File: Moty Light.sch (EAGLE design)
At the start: 14 parts, among them T1 BTA16

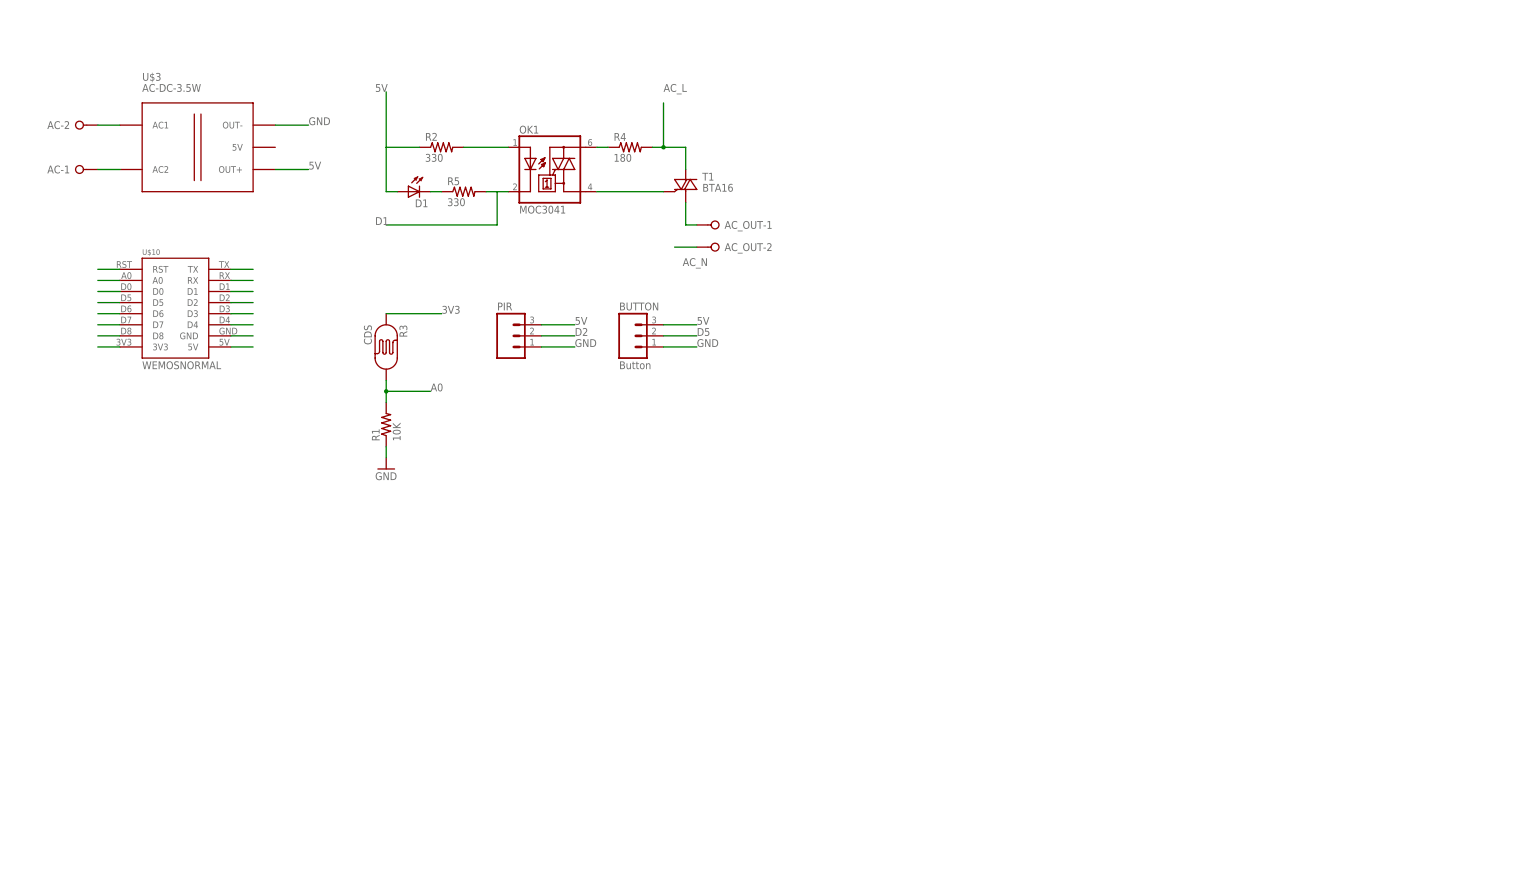
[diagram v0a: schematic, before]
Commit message: Update to version 0.2
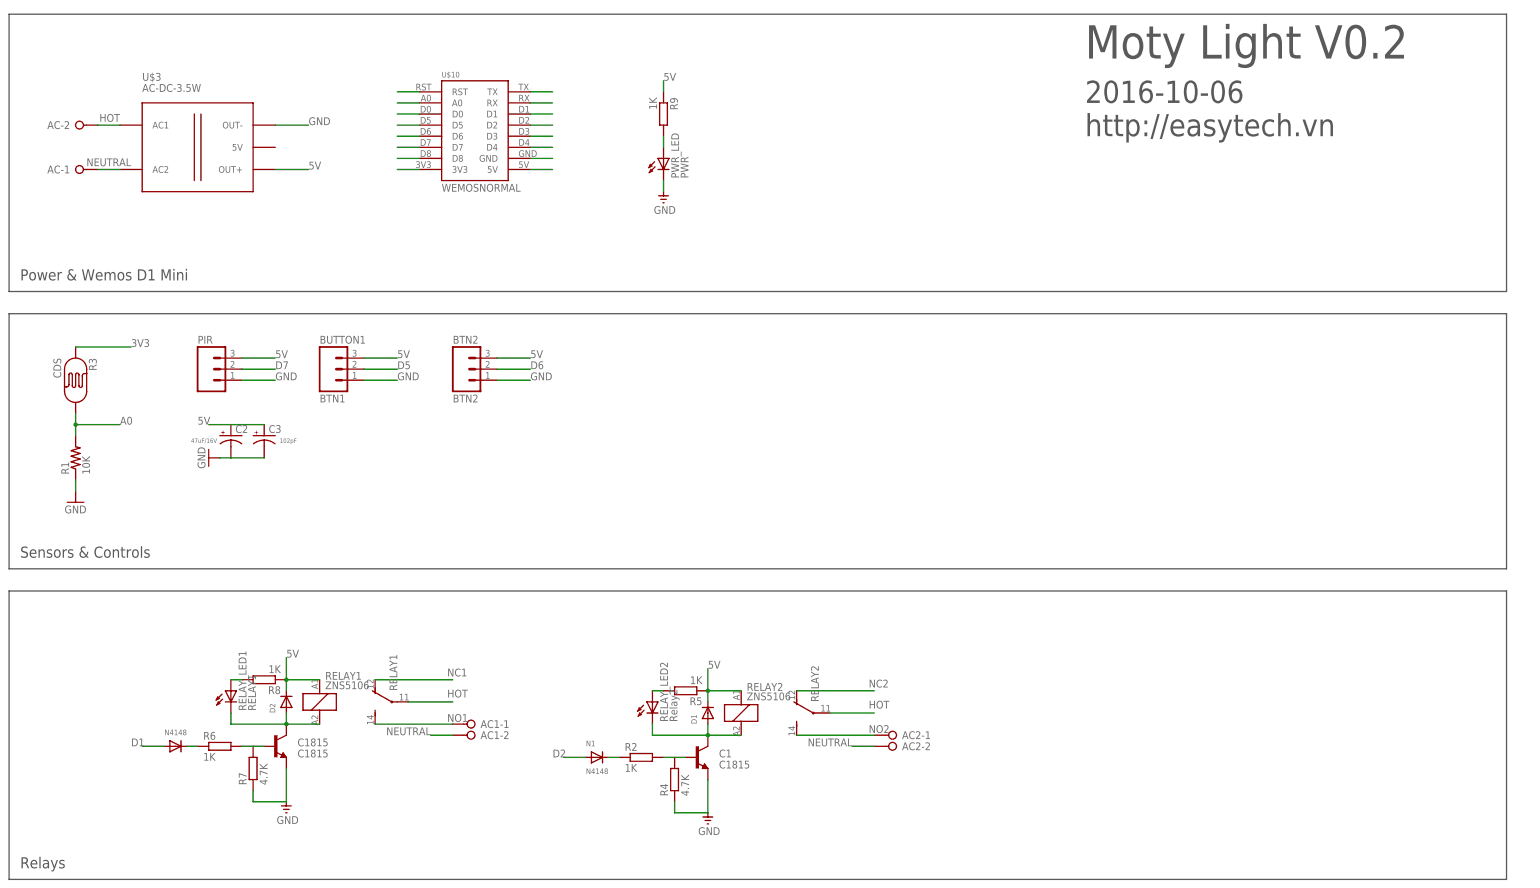
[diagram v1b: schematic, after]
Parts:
- removed AC_OUT: (no value), con-wago-508:W237-02P
- removed BUTTON: Button, SparkFun-Connectors:M03PTH
- removed OK1: MOC3041, optocoupler:MOC3032T
- removed T1: BTA16, triac:BT138-V
- added AC1, AC2: (no value), con-wago-508:W237-02P
- added BTN2: BTN2, SparkFun-Connectors:M03PTH
- added BUTTON1: BTN1, SparkFun-Connectors:M03PTH
- added C1, C1815: C1815, SparkFun-DiscreteSemi:TRANSISTOR_NPNSOT23-3
- added C2: 47uF/16V, SparkFun-Capacitors:CAP_POLPTH2
- added C3: 102pF, SparkFun-Capacitors:CAP_POLPTH2
- added D2: (no value), adafruit:DIODESMA
- added N1: N4148, adafruit:DIODESOD-123
- added N4148: (no value), adafruit:DIODESOD-123
- added PWR_LED: PWR, adafruit:LED3MM
- added R6, R8, R9: 1K, rcl:R-EU_R0805
- added R7: 4.7K, rcl:R-EU_R0805
- added RELAY1, RELAY2: ZNS5106, relay:ZNS5106
- added RELAY_LED1: RELAY1, adafruit:LED3MM
- added RELAY_LED2: Relay2, adafruit:LED3MM
- D1: device led:LED3MM -> adafruit:DIODESMA
- R1: device rcl:R-US_0204/7 -> rcl:R-US_R0805
- R2, R5: value 330 -> 1K; device rcl:R-US_0204/7 -> rcl:R-EU_R0805
- R4: value 180 -> 4.7K; device rcl:R-US_0204/7 -> rcl:R-EU_R0805
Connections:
- removed net AC_L: AC-2.KL, R4.2, T1.A2, U$3.AC1
- removed net AC_N: AC-1.KL, AC_OUT-2.KL, U$3.AC2
- removed net N$14: OK1.A2, R4.1
- removed net N$23: AC_OUT-1.KL, T1.A1
- removed net N$28: D1.C, R5.1
- new net HOT: AC-2.KL, RELAY12.P, RELAY22.P, U$3.AC1
- new net N$1: C1815.C, D2.A, RELAY11.2, RELAY_LED1.C
- new net N$3: N4148.C, R6.1
- new net N$4: R8.2, RELAY_LED1.A
- new net N$5: C1.C, D1.A, RELAY21.2, RELAY_LED2.C
- new net N$6: C1.B, R2.2, R4.2
- new net N$7: C1815.B, R6.2, R7.2
- new net N$8: N1.C, R2.1
- new net NC1: RELAY12.O
- new net NC2: RELAY22.O
- new net NEUTRAL: AC-1.KL, AC1-2.KL, AC2-2.KL, U$3.AC2
- new net NO1: AC1-1.KL, RELAY12.S
- new net NO2: AC2-1.KL, RELAY22.S
- net 5V: now also BTN2.3, BUTTON1.3, C2.+, C3.+, D1.C, D2.C, R5.1, R8.1, R9.1, RELAY11.1, RELAY21.1; no longer BUTTON.3, D1.A, R2.1
- net D1: now also N4148.A; no longer OK1.C, R5.2
- net D2: now also N1.A; no longer PIR.2
- net D5: now also BUTTON1.2; no longer BUTTON.2
- net D6: now also BTN2.2
- net D7: now also PIR.2
- net GND: now also BTN2.1, BUTTON1.1, C1.E, C1815.E, C2.-, C3.-, PWR_LED.C, R4.1, R7.1; no longer BUTTON.1
- net N$10: now also PWR_LED.A, R9.2; no longer OK1.A, R2.2
- net N$9: now also R5.2, RELAY_LED2.A; no longer OK1.A1, T1.G
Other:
- note added: "2016-10-06 http://easytech.vn"
- note added: "Moty Light V0.2"
- note added: "Power & Wemos D1 Mini"
- note added: "Relays"
- note added: "Sensors & Controls"
- moved on the sheet: PIR, R1, R3, U$10

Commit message: Update design to version 0.3
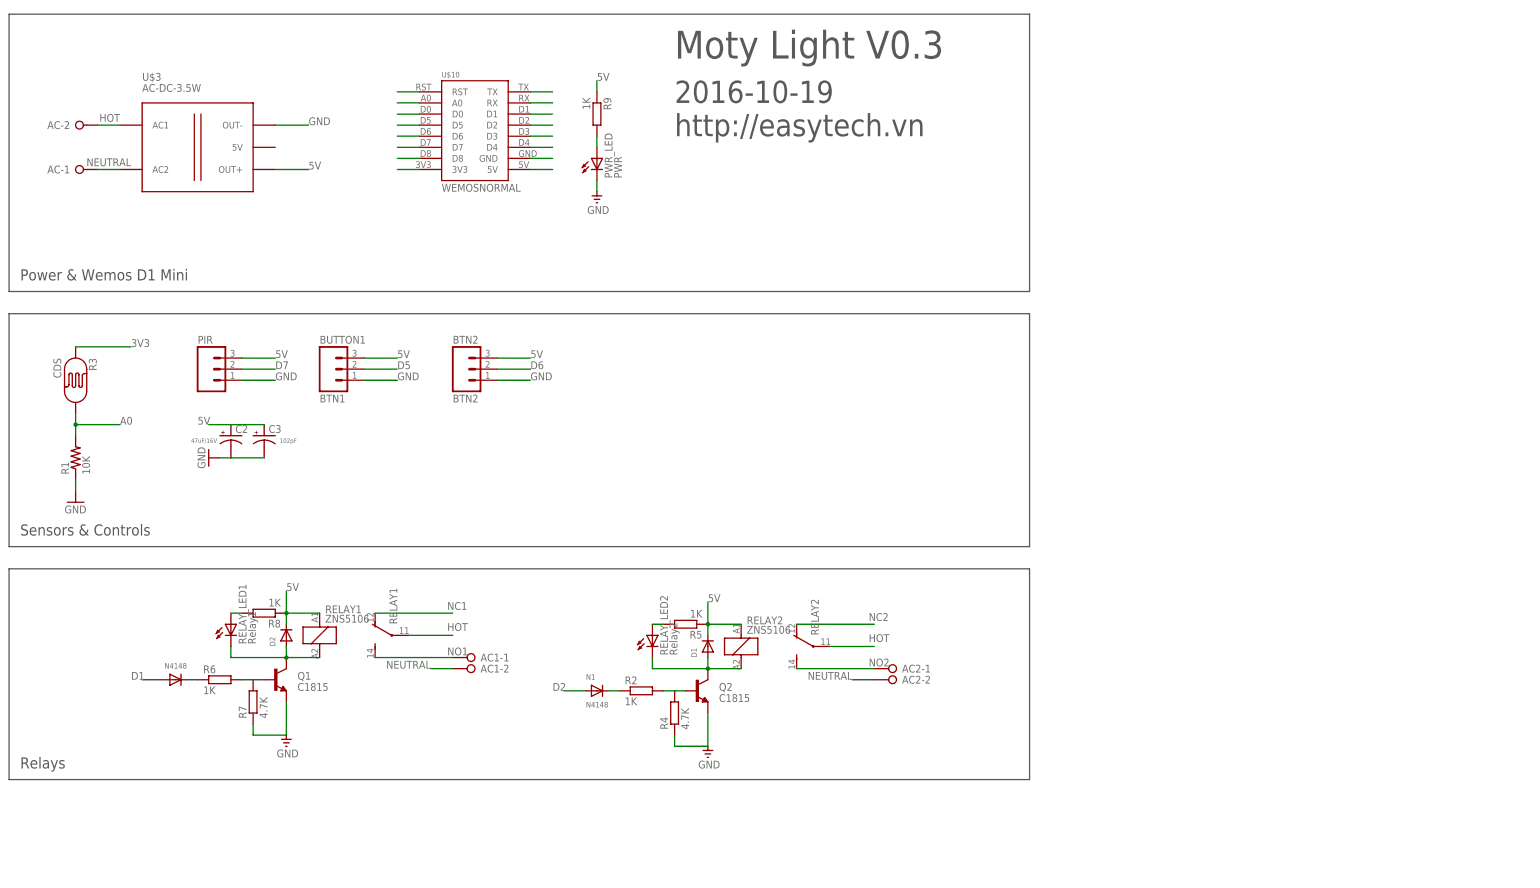
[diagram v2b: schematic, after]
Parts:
- removed C1, C1815: C1815, SparkFun-DiscreteSemi:TRANSISTOR_NPNSOT23-3
- added Q1, Q2: C1815, SparkFun-DiscreteSemi:TRANSISTOR_NPNSOT23-3
- RELAY_LED1: value RELAY1 -> Relay1
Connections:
- net GND: now also Q1.E, Q2.E; no longer C1.E, C1815.E
- net N$1: now also Q1.C; no longer C1815.C
- net N$5: now also Q2.C; no longer C1.C
- net N$6: now also Q2.B; no longer C1.B
- net N$7: now also Q1.B; no longer C1815.B
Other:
- note added: "2016-10-19 http://easytech.vn"
- note added: "Moty Light V0.3"
- note removed: "2016-10-06 http://easytech.vn"
- note removed: "Moty Light V0.2"
- moved on the sheet: AC1-1, AC1-2, AC2-1, AC2-2, D1, D2, N1, N4148, PWR_LED, R2, R4, R5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
